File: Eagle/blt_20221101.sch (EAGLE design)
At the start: 20 parts, among them IC1 74HC4066D, IC2 74HC4066D, IC3 ATTINY84V-10SSUR

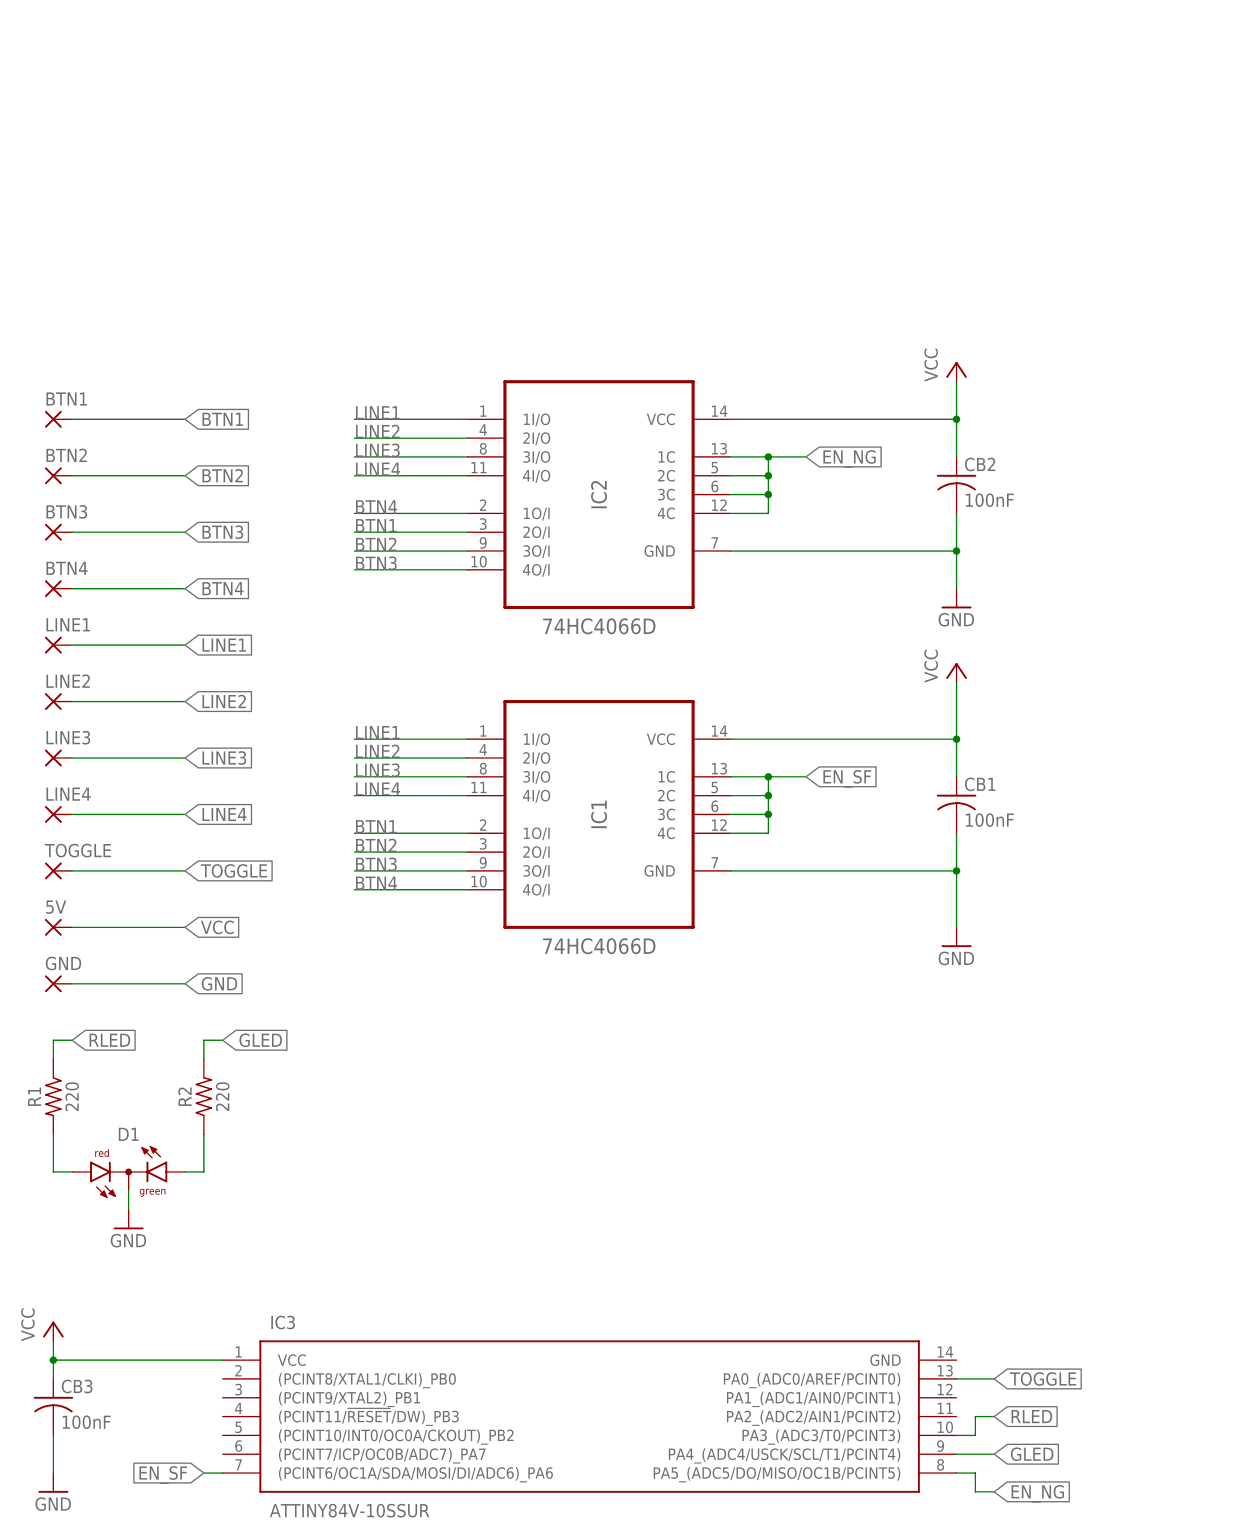
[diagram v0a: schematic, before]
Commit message: Add files via upload
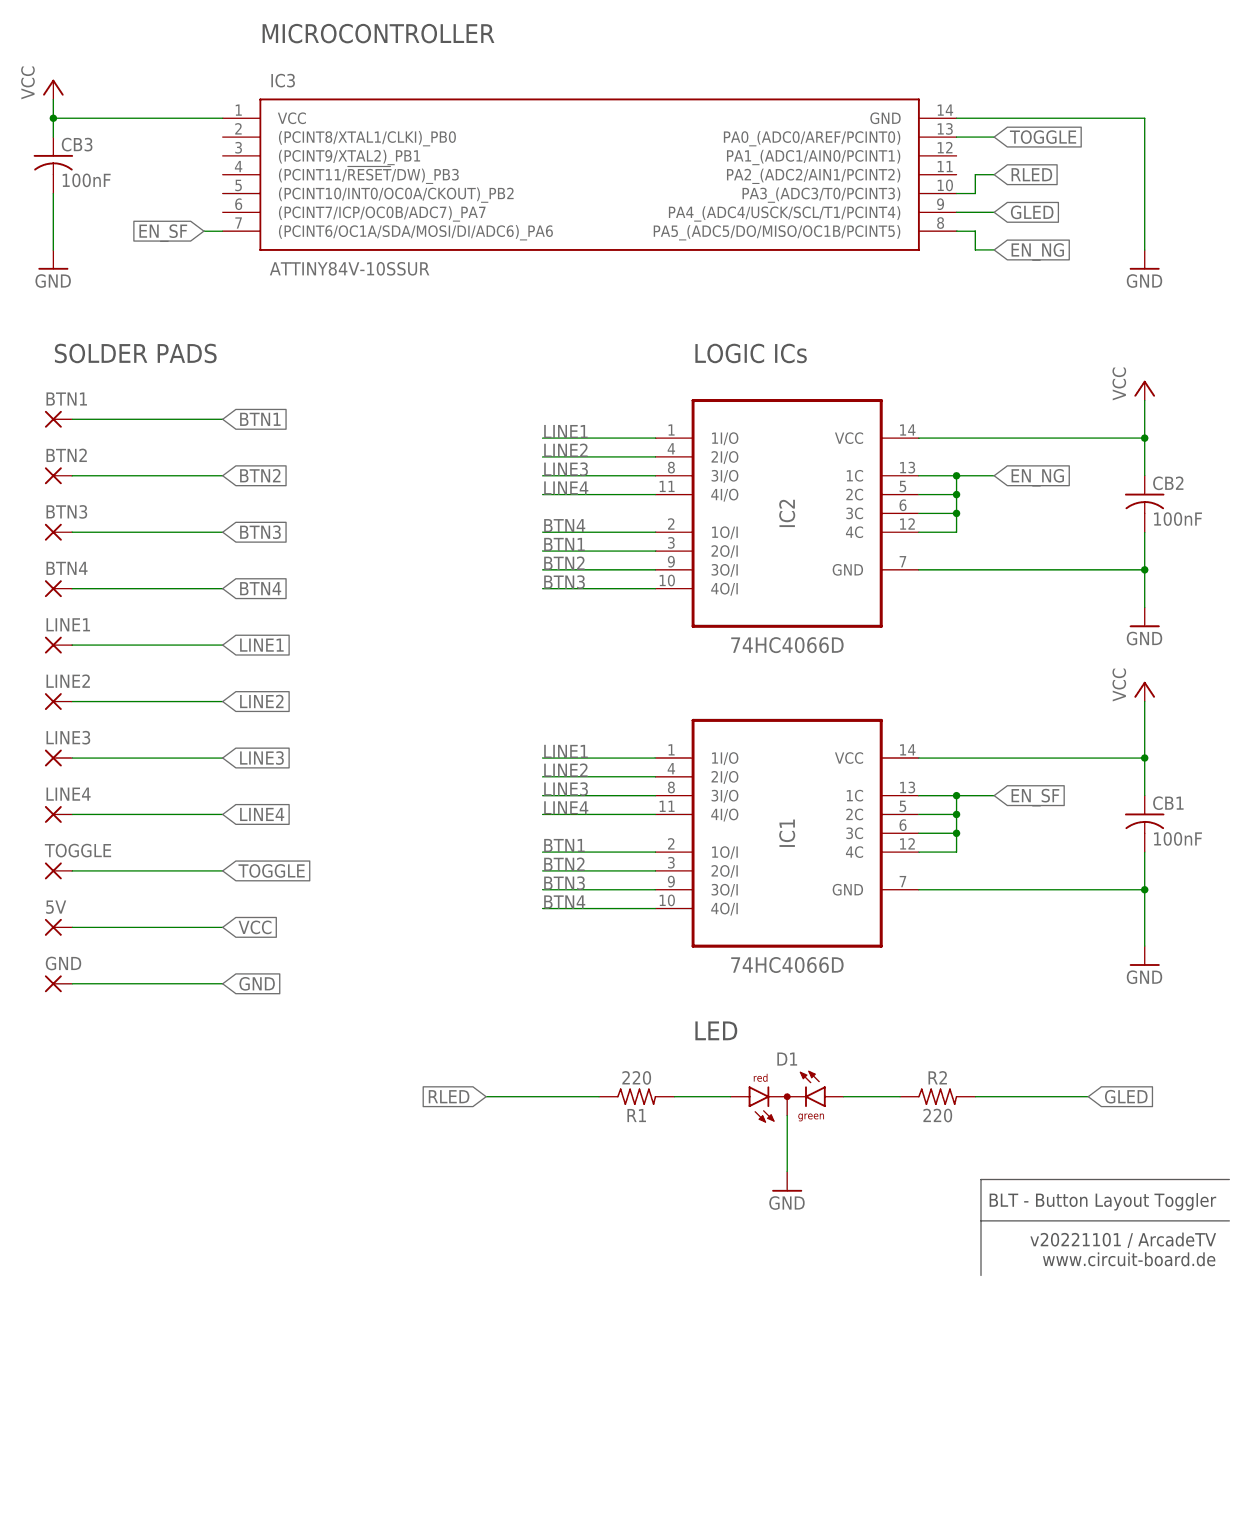
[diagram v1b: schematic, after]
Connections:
- net GND: now also IC3.GND
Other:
- note added: "BLT - Button Layout Toggler v20221101 / ArcadeTV www.circuit-board.de"
- note added: "LED"
- note added: "LOGIC ICs"
- note added: "MICROCONTROLLER"
- note added: "SOLDER PADS"
- moved on the sheet: CB1, CB2, CB3, D1, IC1, IC2, IC3, R1, R2
